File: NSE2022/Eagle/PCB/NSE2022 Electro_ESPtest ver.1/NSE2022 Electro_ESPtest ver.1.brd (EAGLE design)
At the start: 87.6 x 83.8 mm, 60 parts, among them CN1 DM3AT, CON1 FP, CON2 BATT, CON3 SV1, CON4 SV2, CON5 SV3, CON6 SV4, U1 CP2102N-A01-GQFN28

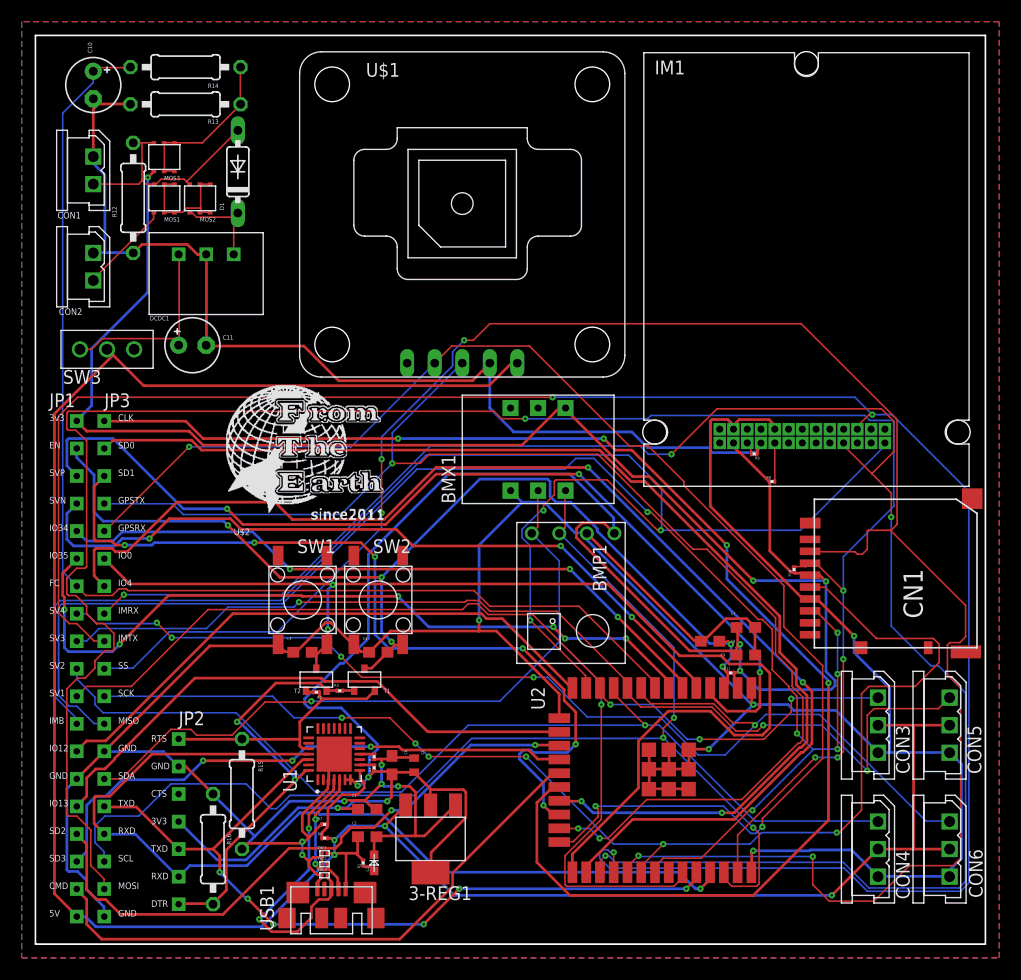
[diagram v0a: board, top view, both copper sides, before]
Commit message: a
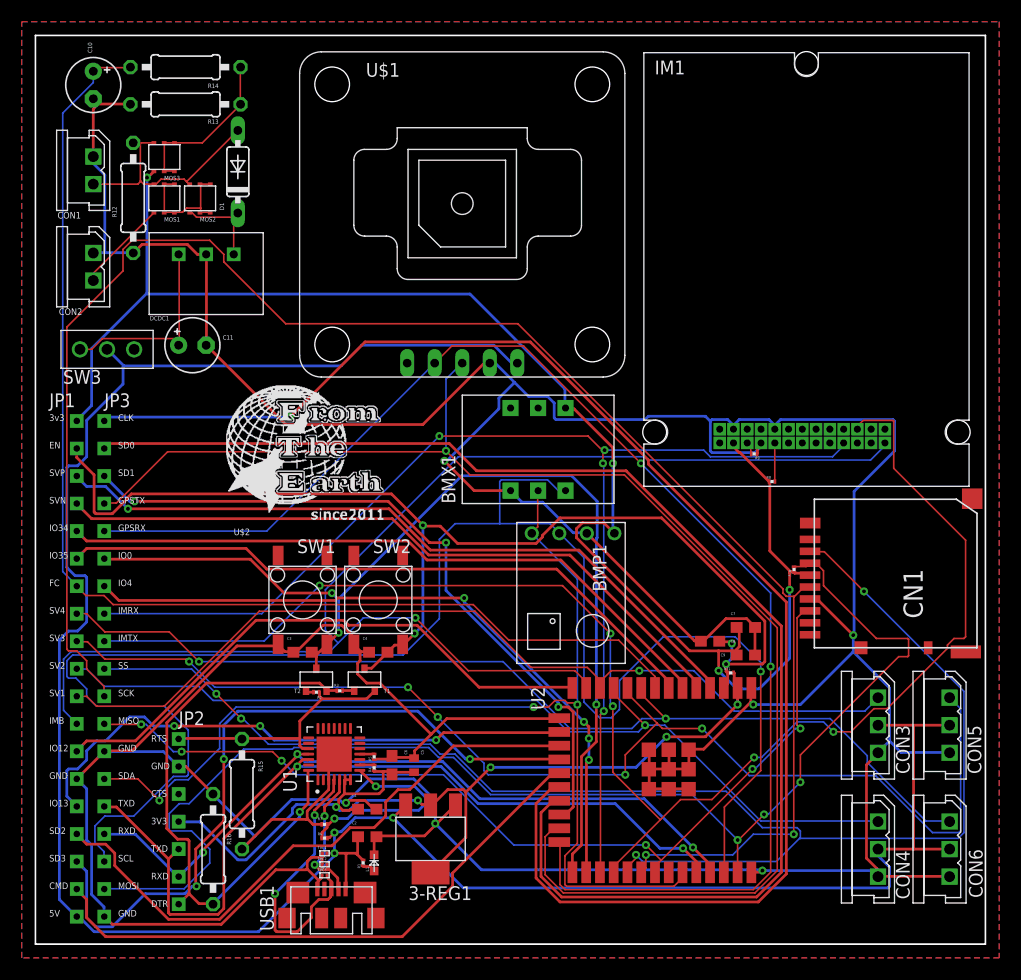
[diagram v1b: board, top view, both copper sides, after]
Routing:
- net MOSI: track 184.8 -> 119.7 mm, vias 5 -> 3
- net IMRX: track 169.4 -> 115.7 mm
- net MISO: track 140.1 -> 87.6 mm
- net IMTX: track 189.4 -> 139.0 mm, vias 3 -> 5
- net IO4: track 114.1 -> 64.0 mm, vias 2 -> 4
- net SS: track 187.0 -> 137.2 mm, vias 5 -> 4
- net SCL: track 110.6 -> 159.1 mm, vias 3 -> 1
- net +3V3: track 280.9 -> 233.7 mm
- net SCK: track 115.1 -> 161.8 mm, vias 6 -> 2
- net GND: track 452.0 -> 491.6 mm, vias 11 -> 6
- net S_VP: track 90.6 -> 66.9 mm, vias 3 -> 1
- net RXD: track 89.0 -> 68.4 mm, vias 1 -> 3
- net DTR: track 38.2 -> 54.7 mm, vias 2 -> 1
- net SD0: track 108.0 -> 124.3 mm, vias 2 -> 0
- net SV3: track 95.4 -> 111.5 mm, vias 3 -> 5
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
